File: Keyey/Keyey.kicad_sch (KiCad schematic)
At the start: 0 parts

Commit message: 22 July update
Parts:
- added A1: RaspberryPi_Pico_W, Module:RaspberryPi_Pico_W_SMD, symbol MCU_Module:RaspberryPi_Pico_W_Extensive
- added D1: Blue, LED_SMD:LED_0805_2012Metric_Pad1.15x1.40mm_HandSolder, symbol Device:LED
- added D10, D11, D12, D13, D14, D15, D16, D17, D18, D19, D2, D20, D21, D22, D23, D24, D25, D26, D27, D28, D29, D3, D30, D31, D32, D33, D34, D35, D36, D37, D38, D39, D40, D41, D42, D43, D44, D45, D46, D47, D48, D49, D50, D51, D52, D53, D54, D55, D56, D57, D58, D59, D6, D60, D61, D62, D63, D64, D65, D66, D67, D69, D70, D71, D74, D75, D76, D78, D79, D8, D80, D82, D83, D84, D85, D86, D87, D88, D89, D9, D90, D91, D92: 1N4148W, Diode_SMD:D_SOD-123, symbol Diode:1N4148W
- added D4: Red, LED_SMD:LED_0805_2012Metric_Pad1.15x1.40mm_HandSolder, symbol Device:LED
- added J1: USB_C_Receptacle_USB2.0_16P, Connector_USB:USB_C_Receptacle_Amphenol_12401948E412A, symbol Connector:USB_C_Receptacle_USB2.0_16P
- added J2: Conn_01x02_Pin, Connector_JST:JST_EH_S2B-EH_1x02_P2.50mm_Horizontal, symbol Connector:Conn_01x02_Pin
- added R1: 5.1K, Resistor_SMD:R_01005_0402Metric_Pad0.57x0.30mm_HandSolder, symbol Device:R
- added R2: 5.1k, Resistor_SMD:R_01005_0402Metric_Pad0.57x0.30mm_HandSolder, symbol Device:R
- added R3, R4: 27, Resistor_SMD:R_01005_0402Metric_Pad0.57x0.30mm_HandSolder, symbol Device:R
- added R5: 1.2K, Resistor_SMD:R_01005_0402Metric_Pad0.57x0.30mm_HandSolder, symbol Device:R
- added R6: 1+, Resistor_SMD:R_01005_0402Metric_Pad0.57x0.30mm_HandSolder, symbol Device:R
- added R7: 1-, Resistor_SMD:R_01005_0402Metric_Pad0.57x0.30mm_HandSolder, symbol Device:R
- added R8: 2+, Resistor_SMD:R_01005_0402Metric_Pad0.57x0.30mm_HandSolder, symbol Device:R
- added R9: 2-, Resistor_SMD:R_01005_0402Metric_Pad0.57x0.30mm_HandSolder, symbol Device:R
- added S1, S3, S4: Stab 2u, PCM_Mounting_Keyboard_Stabilizer:Stabilizer_Cherry_MX_2.00u, symbol PCM_marbastlib-mx:MX_stab
- added S2: Stab 6.25u, PCM_marbastlib-mx:STAB_MX_P_6.25u, symbol PCM_marbastlib-mx:MX_stab
- added SW1: EC11E15244G1, 2026-07-22_12-53-14:EC11E15244G1_AAL, symbol 2026-07-22_12-53-14:EC11E15244G1
- added SW10, SW89: Control, PCM_marbastlib-mx:SW_MX_1u, symbol Switch:SW_Push
- added SW11: F1, PCM_marbastlib-mx:SW_MX_1u, symbol Switch:SW_Push
- added SW12: 1, PCM_marbastlib-mx:SW_MX_1u, symbol Switch:SW_Push
- added SW13: Q, PCM_marbastlib-mx:SW_MX_1u, symbol Switch:SW_Push
- added SW14: A, PCM_marbastlib-mx:SW_MX_1u, symbol Switch:SW_Push
- added SW15: Z, PCM_marbastlib-mx:SW_MX_1u, symbol Switch:SW_Push
- added SW16: Win, PCM_marbastlib-mx:SW_MX_1u, symbol Switch:SW_Push
- added SW17: F2, PCM_marbastlib-mx:SW_MX_1u, symbol Switch:SW_Push
- added SW18: 2, PCM_marbastlib-mx:SW_MX_1u, symbol Switch:SW_Push
- added SW19: W, PCM_marbastlib-mx:SW_MX_1u, symbol Switch:SW_Push
- added SW2: Caplocks, PCM_marbastlib-mx:SW_MX_1u, symbol Switch:SW_Push
- added SW20: S, PCM_marbastlib-mx:SW_MX_1u, symbol Switch:SW_Push
- added SW21: X, PCM_marbastlib-mx:SW_MX_1u, symbol Switch:SW_Push
- added SW22: F3, PCM_marbastlib-mx:SW_MX_1u, symbol Switch:SW_Push
- added SW23: 3, PCM_marbastlib-mx:SW_MX_1u, symbol Switch:SW_Push
- added SW24: E, PCM_marbastlib-mx:SW_MX_1u, symbol Switch:SW_Push
- added SW25: D, PCM_marbastlib-mx:SW_MX_1u, symbol Switch:SW_Push
- added SW26: C, PCM_marbastlib-mx:SW_MX_1u, symbol Switch:SW_Push
- added SW27: F4, PCM_marbastlib-mx:SW_MX_1u, symbol Switch:SW_Push
- added SW28: 4, PCM_marbastlib-mx:SW_MX_1u, symbol Switch:SW_Push
- added SW29: R, PCM_marbastlib-mx:SW_MX_1u, symbol Switch:SW_Push
- added SW30: F, PCM_marbastlib-mx:SW_MX_1u, symbol Switch:SW_Push
- added SW31: V, PCM_marbastlib-mx:SW_MX_1u, symbol Switch:SW_Push
- added SW32, SW80: opt, PCM_marbastlib-mx:SW_MX_1u, symbol Switch:SW_Push
- added SW33: F5, PCM_marbastlib-mx:SW_MX_1u, symbol Switch:SW_Push
- added SW34: 5, PCM_marbastlib-mx:SW_MX_1u, symbol Switch:SW_Push
- added SW35: T, PCM_marbastlib-mx:SW_MX_1u, symbol Switch:SW_Push
- added SW36: G, PCM_marbastlib-mx:SW_MX_1u, symbol Switch:SW_Push
- added SW37: B, PCM_marbastlib-mx:SW_MX_1u, symbol Switch:SW_Push
- added SW38: F6, PCM_marbastlib-mx:SW_MX_1u, symbol Switch:SW_Push
- added SW39: 6, PCM_marbastlib-mx:SW_MX_1u, symbol Switch:SW_Push
- added SW4: Tab, PCM_marbastlib-mx:SW_MX_1u, symbol Switch:SW_Push
- added SW40: Y, PCM_marbastlib-mx:SW_MX_1u, symbol Switch:SW_Push
- added SW41: H, PCM_marbastlib-mx:SW_MX_1u, symbol Switch:SW_Push
- added SW42: N, PCM_marbastlib-mx:SW_MX_1u, symbol Switch:SW_Push
- added SW43: F7, PCM_marbastlib-mx:SW_MX_1u, symbol Switch:SW_Push
- added SW44: 7, PCM_marbastlib-mx:SW_MX_1u, symbol Switch:SW_Push
- added SW45: U, PCM_marbastlib-mx:SW_MX_1u, symbol Switch:SW_Push
- added SW46: J, PCM_marbastlib-mx:SW_MX_1u, symbol Switch:SW_Push
- added SW47: M, PCM_marbastlib-mx:SW_MX_1u, symbol Switch:SW_Push
- added SW48: Spacebar, PCM_marbastlib-mx:SW_MX_1u, symbol Switch:SW_Push
- added SW49: F8, PCM_marbastlib-mx:SW_MX_1u, symbol Switch:SW_Push
- added SW5: Left Shift, PCM_marbastlib-mx:SW_MX_1u, symbol Switch:SW_Push
- added SW50: 8, PCM_marbastlib-mx:SW_MX_1u, symbol Switch:SW_Push
- added SW51: I, PCM_marbastlib-mx:SW_MX_1u, symbol Switch:SW_Push
- added SW52: K, PCM_marbastlib-mx:SW_MX_1u, symbol Switch:SW_Push
- added SW53: ,, PCM_marbastlib-mx:SW_MX_1u, symbol Switch:SW_Push
- added SW54: F9, PCM_marbastlib-mx:SW_MX_1u, symbol Switch:SW_Push
- added SW55: 9, PCM_marbastlib-mx:SW_MX_1u, symbol Switch:SW_Push
- added SW56: O, PCM_marbastlib-mx:SW_MX_1u, symbol Switch:SW_Push
- added SW57: L, PCM_marbastlib-mx:SW_MX_1u, symbol Switch:SW_Push
- added SW58: ., PCM_marbastlib-mx:SW_MX_1u, symbol Switch:SW_Push
- added SW59: F10, PCM_marbastlib-mx:SW_MX_1u, symbol Switch:SW_Push
- added SW60: 0, PCM_marbastlib-mx:SW_MX_1u, symbol Switch:SW_Push
- added SW61: P, PCM_marbastlib-mx:SW_MX_1u, symbol Switch:SW_Push
- added SW62: ;, PCM_marbastlib-mx:SW_MX_1u, symbol Switch:SW_Push
- added SW63: /, PCM_marbastlib-mx:SW_MX_1u, symbol Switch:SW_Push
- added SW64: F11, PCM_marbastlib-mx:SW_MX_1u, symbol Switch:SW_Push
- added SW65: -, PCM_marbastlib-mx:SW_MX_1u, symbol Switch:SW_Push
- added SW66: [, PCM_marbastlib-mx:SW_MX_1u, symbol Switch:SW_Push
- added SW67: ', PCM_marbastlib-mx:SW_MX_1u, symbol Switch:SW_Push
- added SW69: F12, PCM_marbastlib-mx:SW_MX_1u, symbol Switch:SW_Push
- added SW70: =, PCM_marbastlib-mx:SW_MX_1u, symbol Switch:SW_Push
- added SW71: ], PCM_marbastlib-mx:SW_MX_1u, symbol Switch:SW_Push
- added SW74: prntsrc, PCM_marbastlib-mx:SW_MX_1u, symbol Switch:SW_Push
- added SW75: backspace, PCM_marbastlib-mx:SW_MX_1u, symbol Switch:SW_Push
- added SW76: \, PCM_marbastlib-mx:SW_MX_1u, symbol Switch:SW_Push
- added SW78: SHIFT, PCM_marbastlib-mx:SW_MX_1u, symbol Switch:SW_Push
- added SW79: del, PCM_marbastlib-mx:SW_MX_1u, symbol Switch:SW_Push
- added SW8: Esc, PCM_marbastlib-mx:SW_MX_1u, symbol Switch:SW_Push
- added SW82: ENTER, PCM_marbastlib-mx:SW_MX_1u, symbol Switch:SW_Push
- added SW83: up, PCM_marbastlib-mx:SW_MX_1u, symbol Switch:SW_Push
- added SW84: fn, PCM_marbastlib-mx:SW_MX_1u, symbol Switch:SW_Push
- added SW85: pgup, PCM_marbastlib-mx:SW_MX_1u, symbol Switch:SW_Push
- added SW86: pgdn, PCM_marbastlib-mx:SW_MX_1u, symbol Switch:SW_Push
- added SW87: home, PCM_marbastlib-mx:SW_MX_1u, symbol Switch:SW_Push
- added SW88: end, PCM_marbastlib-mx:SW_MX_1u, symbol Switch:SW_Push
- added SW9: ~, PCM_marbastlib-mx:SW_MX_1u, symbol Switch:SW_Push
- added SW90: left, PCM_marbastlib-mx:SW_MX_1u, symbol Switch:SW_Push
- added SW91: down, PCM_marbastlib-mx:SW_MX_1u, symbol Switch:SW_Push
- added SW92: right, PCM_marbastlib-mx:SW_MX_1u, symbol Switch:SW_Push
- added U1: TP4056, Package_SO:SOP-8-1EP_4.57x4.57mm_P1.27mm_EP4.57x4.45mm, symbol PCM_marbastlib-various:TP4056
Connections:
- new net: D91.2 (A), SW91.2
- new net: D24.2 (A), SW24.2
- new net: D29.2 (A), SW29.2
- new net: D46.2 (A), SW46.2
- new net: D89.2 (A), SW89.2
- new net: D83.2 (A), SW83.2
- new net: D90.2 (A), SW90.2
- new net: D65.2 (A), SW65.2
- new net: D70.2 (A), SW70.2
- new net: D15.2 (A), SW15.2
- new net: D82.2 (A), SW82.2
- new net: D14.2 (A), SW14.2
- new net: D76.2 (A), SW76.2
- new net: D10.2 (A), SW10.2
- new net: D26.2 (A), SW26.2
- new net: D42.2 (A), SW42.2
- new net: D37.2 (A), SW37.2
- new net: D39.2 (A), SW39.2
- new net: D6.2 (A), SW4.2
- new net: D13.2 (A), SW13.2
- new net: D87.2 (A), SW87.2
- new net: D51.2 (A), SW51.2
- new net: D12.2 (A), SW12.2
- new net: D20.2 (A), SW20.2
- new net: D11.2 (A), SW11.2
- new net: D22.2 (A), SW22.2
- new net: D57.2 (A), SW57.2
- new net: D48.2 (A), SW48.2
- new net: D80.2 (A), SW80.2
- new net: D85.2 (A), SW85.2
- new net: D21.2 (A), SW21.2
- new net: D67.2 (A), SW67.2
- new net: D36.2 (A), SW36.2
- new net: D50.2 (A), SW50.2
- new net: D9.2 (A), SW9.2
- new net: D55.2 (A), SW55.2
- new net: D64.2 (A), SW64.2
- new net: D2.2 (A), SW2.2
- new net: D17.2 (A), SW17.2
- new net: A1.40 (VBUS), J1.A4 (VBUS), J1.A9 (VBUS), J1.B4 (VBUS), J1.B9 (VBUS)
- new net: A1.TP2 (USB_DM), J1.A7 (D-), J1.B7 (D-), R3.2
- new net: A1.TP3 (USB_DP), J1.A6 (D+), J1.B6 (D+), R4.2
- new net: J1.B5 (CC2), R2.1
- new net: D66.2 (A), SW66.2
- new net: D79.2 (A), SW79.2
- new net: D75.2 (A), SW75.2
- new net: D23.2 (A), SW23.2
- new net: D88.2 (A), SW88.2
- new net: D61.2 (A), SW61.2
- new net: D71.2 (A), SW71.2
- new net: D31.2 (A), SW31.2
- new net: D25.2 (A), SW25.2
- new net: D30.2 (A), SW30.2
- new net: D18.2 (A), SW18.2
- new net: D8.2 (A), SW8.2
- new net: D33.2 (A), SW33.2
- new net: D54.2 (A), SW54.2
- new net: J2.1 (Pin_1), R6.1, R7.1
- new net: J2.2 (Pin_2), R8.2, R9.2
- new net: D62.2 (A), SW62.2
- new net: D86.2 (A), SW86.2
- new net: D19.2 (A), SW19.2
- new net: D32.2 (A), SW32.2
- new net: D43.2 (A), SW43.2
- new net: D40.2 (A), SW40.2
- new net: J1.A5 (CC1), R1.1
- new net: D53.2 (A), SW53.2
- new net: D35.2 (A), SW35.2
- new net: D34.2 (A), SW34.2
- new net: D3.2 (A), SW5.2
- new net: D58.2 (A), SW58.2
- new net: D60.2 (A), SW60.2
- new net: D52.2 (A), SW52.2
- new net: R6.2, R8.1, U1.5 (BAT)
- new net: D74.2 (A), SW74.2
- new net: R5.1, U1.2 (PROG)
- new net: D45.2 (A), SW45.2
- new net: D69.2 (A), SW69.2
- new net: D38.2 (A), SW38.2
- new net: D56.2 (A), SW56.2
- new net: D84.2 (A), SW84.2
- new net: R7.2, R9.1, U1.1 (TEMP)
- new net: D28.2 (A), SW28.2
- new net: D41.2 (A), SW41.2
- new net: D59.2 (A), SW59.2
- new net: D63.2 (A), SW63.2
- new net: D16.2 (A), SW16.2
- new net: D78.2 (A), SW78.2
- new net: D49.2 (A), SW49.2
- new net: D27.2 (A), SW27.2
- new net: D92.2 (A), SW92.2
- new net: D44.2 (A), SW44.2
- new net: D47.2 (A), SW47.2
- new net COL1: SW10.1, SW2.1, SW4.1, SW5.1, SW8.1, SW9.1
- new net COL10: SW54.1, SW55.1, SW56.1, SW57.1, SW58.1, SW80.1
- new net COL11: SW59.1, SW60.1, SW61.1, SW62.1, SW63.1, SW84.1
- new net COL12: SW64.1, SW65.1, SW66.1, SW67.1, SW78.1, SW90.1
- new net COL13: SW69.1, SW70.1, SW71.1, SW82.1, SW83.1, SW91.1
- new net COL14: SW74.1, SW75.1, SW76.1
- new net COL15: SW79.1, SW85.1, SW86.1, SW87.1, SW88.1, SW92.1
- new net COL2: SW11.1, SW12.1, SW13.1, SW14.1, SW15.1, SW16.1
- new net COL3: SW17.1, SW18.1, SW19.1, SW20.1, SW21.1, SW32.1
- new net COL4: SW22.1, SW23.1, SW24.1, SW25.1, SW26.1
- new net COL5: SW27.1, SW28.1, SW29.1, SW30.1, SW31.1
- new net COL6: SW33.1, SW34.1, SW35.1, SW36.1, SW37.1
- new net COL7: SW38.1, SW39.1, SW40.1, SW41.1, SW42.1
- new net COL8: SW43.1, SW44.1, SW45.1, SW46.1, SW47.1
- new net COL9: SW49.1, SW50.1, SW51.1, SW52.1, SW53.1
- new net GND: A1.13 (GND), A1.18 (GND), A1.23 (GND), A1.28 (GND), A1.3 (GND), A1.33 (AGND), A1.38 (GND), A1.8 (GND), A1.D2 (GND), A1.TP1 (USB_GND), J1.A1 (GND), J1.A12 (GND), J1.B1 (GND), J1.B12 (GND), J1.SH (SHIELD), R1.2, R2.2, R3.1, R4.1, R5.2
- new net ROW1: D11.1 (K), D17.1 (K), D22.1 (K), D27.1 (K), D33.1 (K), D38.1 (K), D43.1 (K), D49.1 (K), D54.1 (K), D59.1 (K), D64.1 (K), D69.1 (K), D74.1 (K), D79.1 (K), D8.1 (K)
- new net ROW2: D12.1 (K), D18.1 (K), D23.1 (K), D28.1 (K), D34.1 (K), D39.1 (K), D44.1 (K), D50.1 (K), D55.1 (K), D60.1 (K), D65.1 (K), D70.1 (K), D75.1 (K), D85.1 (K), D9.1 (K)
- new net ROW3: D13.1 (K), D19.1 (K), D24.1 (K), D29.1 (K), D35.1 (K), D40.1 (K), D45.1 (K), D51.1 (K), D56.1 (K), D6.1 (K), D61.1 (K), D66.1 (K), D71.1 (K), D76.1 (K), D86.1 (K)
- new net ROW4: D14.1 (K), D2.1 (K), D20.1 (K), D25.1 (K), D30.1 (K), D36.1 (K), D41.1 (K), D46.1 (K), D52.1 (K), D57.1 (K), D62.1 (K), D67.1 (K), D82.1 (K), D87.1 (K)
- new net ROW5: D15.1 (K), D21.1 (K), D26.1 (K), D3.1 (K), D31.1 (K), D37.1 (K), D42.1 (K), D47.1 (K), D53.1 (K), D58.1 (K), D63.1 (K), D83.1 (K), D88.1 (K)
- new net ROW6: D10.1 (K), D16.1 (K), D32.1 (K), D48.1 (K), D80.1 (K), D84.1 (K), D89.1 (K), D90.1 (K), D91.1 (K), D92.1 (K)

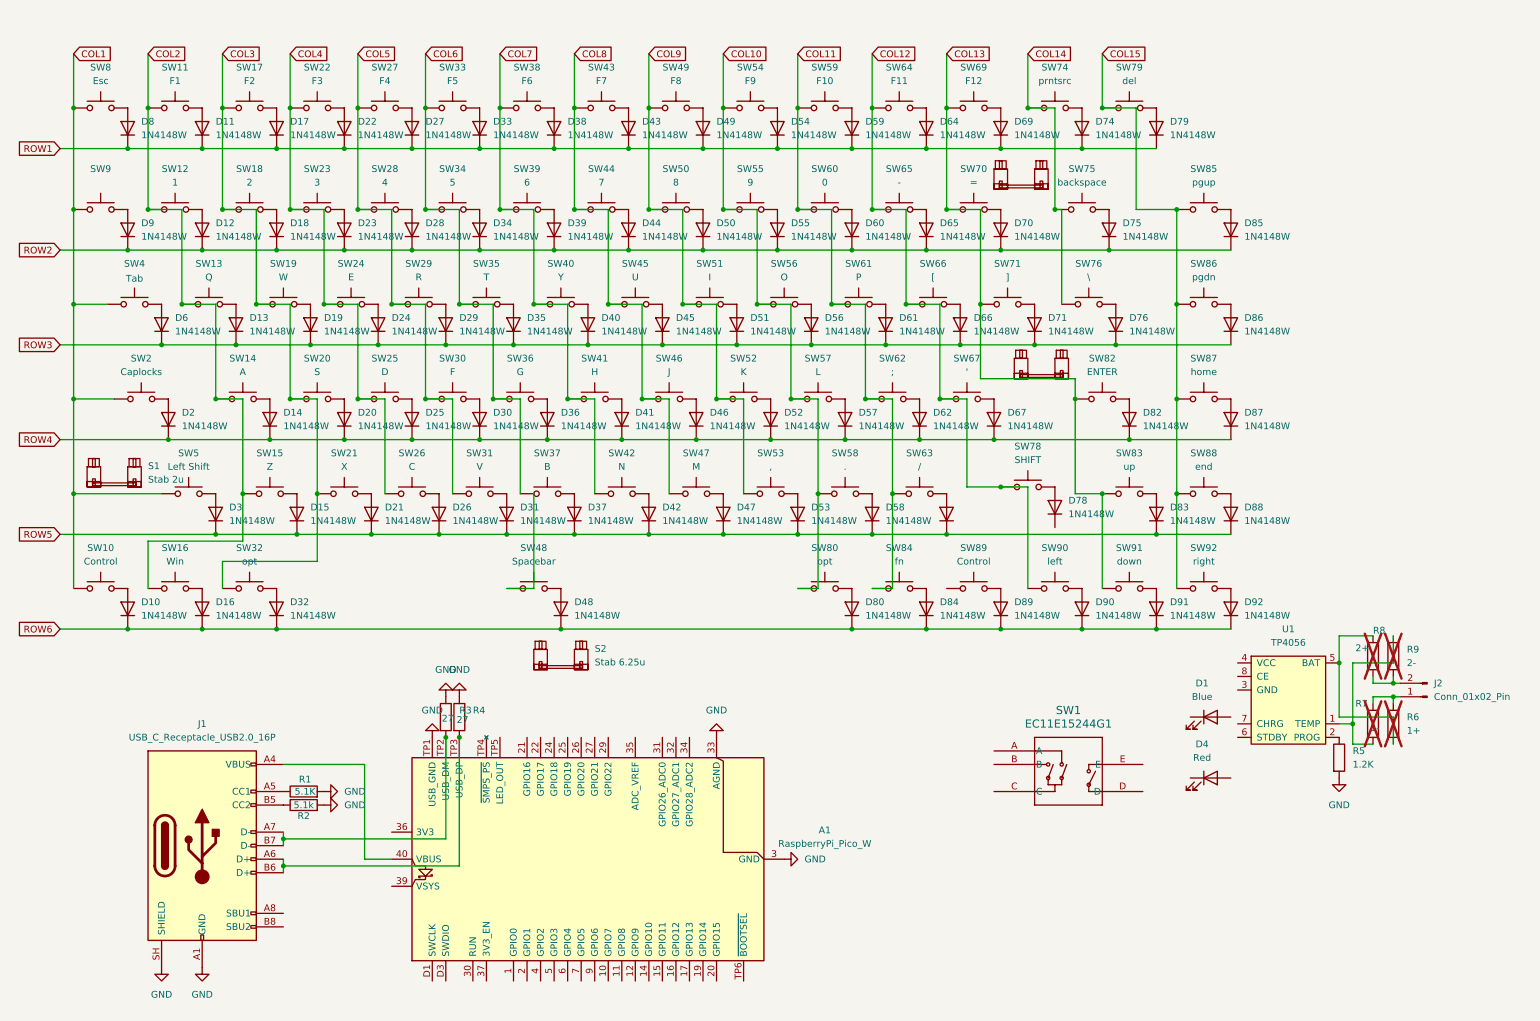
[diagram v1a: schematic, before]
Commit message: July 23-25 update
More info check: https://stardance.hackclub.com/projects/10369
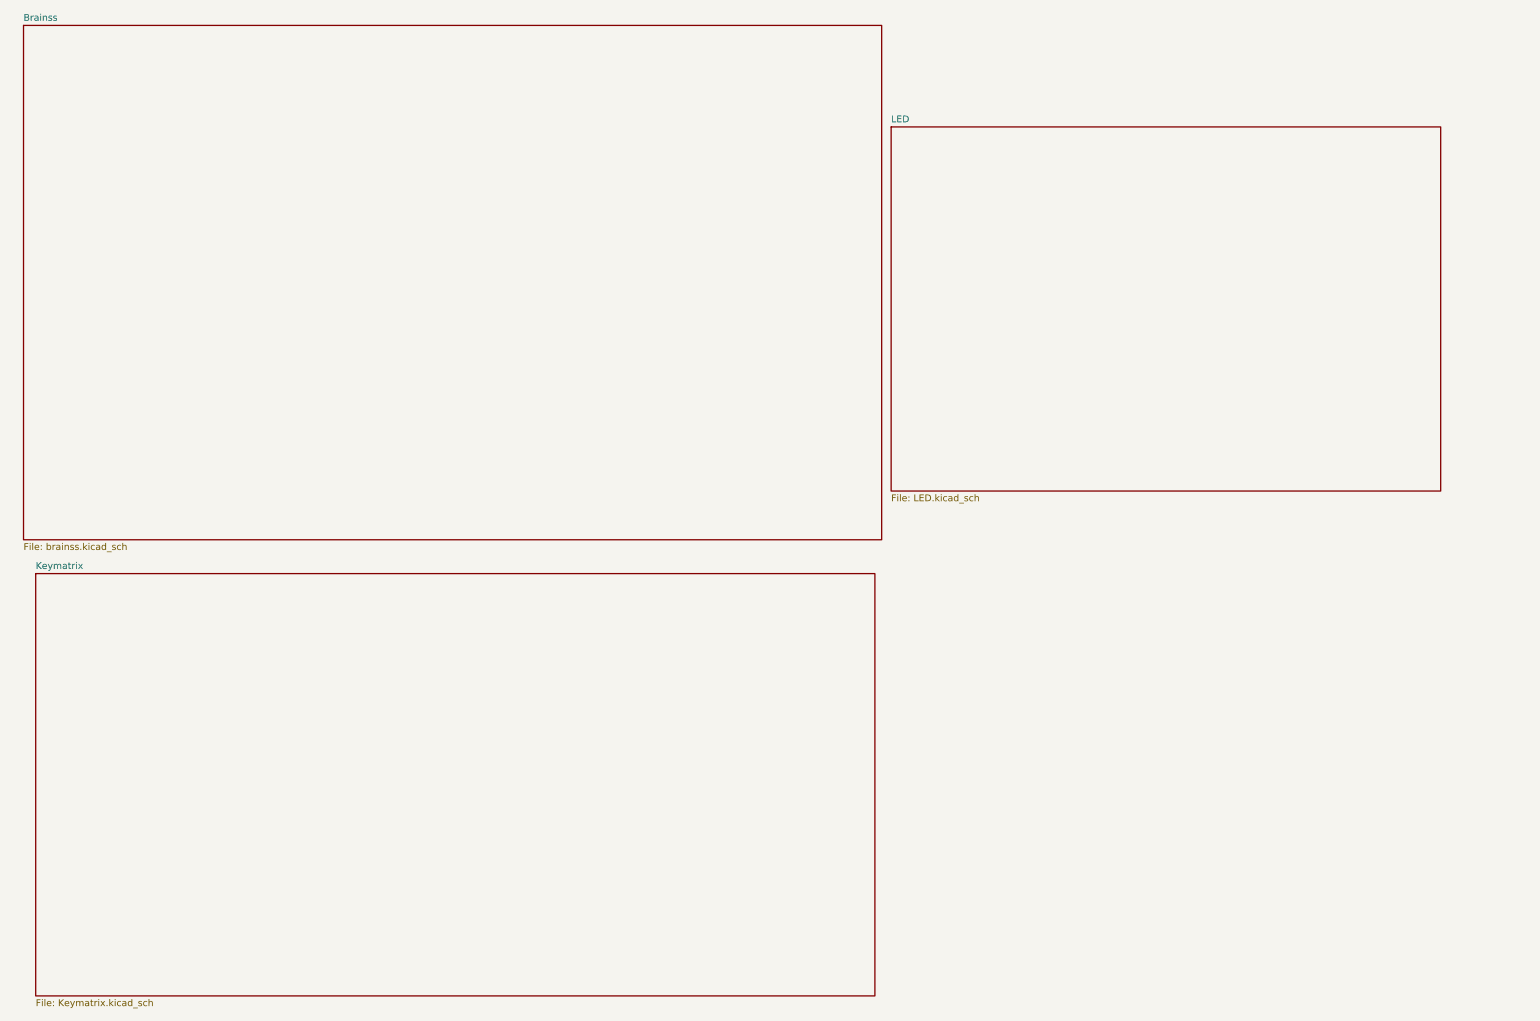
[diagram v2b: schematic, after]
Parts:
- removed A1: RaspberryPi_Pico_W, Module:RaspberryPi_Pico_W_SMD, symbol MCU_Module:RaspberryPi_Pico_W_Extensive
- removed D1: Blue, LED_SMD:LED_0805_2012Metric_Pad1.15x1.40mm_HandSolder, symbol Device:LED
- removed D10, D11, D12, D13, D14, D15, D16, D17, D18, D19, D2, D20, D21, D22, D23, D24, D25, D26, D27, D28, D29, D3, D30, D31, D32, D33, D34, D35, D36, D37, D38, D39, D40, D41, D42, D43, D44, D45, D46, D47, D48, D49, D50, D51, D52, D53, D54, D55, D56, D57, D58, D59, D6, D60, D61, D62, D63, D64, D65, D66, D67, D69, D70, D71, D74, D75, D76, D78, D79, D8, D80, D82, D83, D84, D85, D86, D87, D88, D89, D9, D90, D91, D92: 1N4148W, Diode_SMD:D_SOD-123, symbol Diode:1N4148W
- removed D4: Red, LED_SMD:LED_0805_2012Metric_Pad1.15x1.40mm_HandSolder, symbol Device:LED
- removed J1: USB_C_Receptacle_USB2.0_16P, Connector_USB:USB_C_Receptacle_Amphenol_12401948E412A, symbol Connector:USB_C_Receptacle_USB2.0_16P
- removed J2: Conn_01x02_Pin, Connector_JST:JST_EH_S2B-EH_1x02_P2.50mm_Horizontal, symbol Connector:Conn_01x02_Pin
- removed R1: 5.1K, Resistor_SMD:R_01005_0402Metric_Pad0.57x0.30mm_HandSolder, symbol Device:R
- removed R2: 5.1k, Resistor_SMD:R_01005_0402Metric_Pad0.57x0.30mm_HandSolder, symbol Device:R
- removed R3, R4: 27, Resistor_SMD:R_01005_0402Metric_Pad0.57x0.30mm_HandSolder, symbol Device:R
- removed R5: 1.2K, Resistor_SMD:R_01005_0402Metric_Pad0.57x0.30mm_HandSolder, symbol Device:R
- removed R6: 1+, Resistor_SMD:R_01005_0402Metric_Pad0.57x0.30mm_HandSolder, symbol Device:R
- removed R7: 1-, Resistor_SMD:R_01005_0402Metric_Pad0.57x0.30mm_HandSolder, symbol Device:R
- removed R8: 2+, Resistor_SMD:R_01005_0402Metric_Pad0.57x0.30mm_HandSolder, symbol Device:R
- removed R9: 2-, Resistor_SMD:R_01005_0402Metric_Pad0.57x0.30mm_HandSolder, symbol Device:R
- removed S1, S3, S4: Stab 2u, PCM_Mounting_Keyboard_Stabilizer:Stabilizer_Cherry_MX_2.00u, symbol PCM_marbastlib-mx:MX_stab
- removed S2: Stab 6.25u, PCM_marbastlib-mx:STAB_MX_P_6.25u, symbol PCM_marbastlib-mx:MX_stab
- removed SW1: EC11E15244G1, 2026-07-22_12-53-14:EC11E15244G1_AAL, symbol 2026-07-22_12-53-14:EC11E15244G1
- removed SW10, SW89: Control, PCM_marbastlib-mx:SW_MX_1u, symbol Switch:SW_Push
- removed SW11: F1, PCM_marbastlib-mx:SW_MX_1u, symbol Switch:SW_Push
- removed SW12: 1, PCM_marbastlib-mx:SW_MX_1u, symbol Switch:SW_Push
- removed SW13: Q, PCM_marbastlib-mx:SW_MX_1u, symbol Switch:SW_Push
- removed SW14: A, PCM_marbastlib-mx:SW_MX_1u, symbol Switch:SW_Push
- removed SW15: Z, PCM_marbastlib-mx:SW_MX_1u, symbol Switch:SW_Push
- removed SW16: Win, PCM_marbastlib-mx:SW_MX_1u, symbol Switch:SW_Push
- removed SW17: F2, PCM_marbastlib-mx:SW_MX_1u, symbol Switch:SW_Push
- removed SW18: 2, PCM_marbastlib-mx:SW_MX_1u, symbol Switch:SW_Push
- removed SW19: W, PCM_marbastlib-mx:SW_MX_1u, symbol Switch:SW_Push
- removed SW2: Caplocks, PCM_marbastlib-mx:SW_MX_1u, symbol Switch:SW_Push
- removed SW20: S, PCM_marbastlib-mx:SW_MX_1u, symbol Switch:SW_Push
- removed SW21: X, PCM_marbastlib-mx:SW_MX_1u, symbol Switch:SW_Push
- removed SW22: F3, PCM_marbastlib-mx:SW_MX_1u, symbol Switch:SW_Push
- removed SW23: 3, PCM_marbastlib-mx:SW_MX_1u, symbol Switch:SW_Push
- removed SW24: E, PCM_marbastlib-mx:SW_MX_1u, symbol Switch:SW_Push
- removed SW25: D, PCM_marbastlib-mx:SW_MX_1u, symbol Switch:SW_Push
- removed SW26: C, PCM_marbastlib-mx:SW_MX_1u, symbol Switch:SW_Push
- removed SW27: F4, PCM_marbastlib-mx:SW_MX_1u, symbol Switch:SW_Push
- removed SW28: 4, PCM_marbastlib-mx:SW_MX_1u, symbol Switch:SW_Push
- removed SW29: R, PCM_marbastlib-mx:SW_MX_1u, symbol Switch:SW_Push
- removed SW30: F, PCM_marbastlib-mx:SW_MX_1u, symbol Switch:SW_Push
- removed SW31: V, PCM_marbastlib-mx:SW_MX_1u, symbol Switch:SW_Push
- removed SW32, SW80: opt, PCM_marbastlib-mx:SW_MX_1u, symbol Switch:SW_Push
- removed SW33: F5, PCM_marbastlib-mx:SW_MX_1u, symbol Switch:SW_Push
- removed SW34: 5, PCM_marbastlib-mx:SW_MX_1u, symbol Switch:SW_Push
- removed SW35: T, PCM_marbastlib-mx:SW_MX_1u, symbol Switch:SW_Push
- removed SW36: G, PCM_marbastlib-mx:SW_MX_1u, symbol Switch:SW_Push
- removed SW37: B, PCM_marbastlib-mx:SW_MX_1u, symbol Switch:SW_Push
- removed SW38: F6, PCM_marbastlib-mx:SW_MX_1u, symbol Switch:SW_Push
- removed SW39: 6, PCM_marbastlib-mx:SW_MX_1u, symbol Switch:SW_Push
- removed SW4: Tab, PCM_marbastlib-mx:SW_MX_1u, symbol Switch:SW_Push
- removed SW40: Y, PCM_marbastlib-mx:SW_MX_1u, symbol Switch:SW_Push
- removed SW41: H, PCM_marbastlib-mx:SW_MX_1u, symbol Switch:SW_Push
- removed SW42: N, PCM_marbastlib-mx:SW_MX_1u, symbol Switch:SW_Push
- removed SW43: F7, PCM_marbastlib-mx:SW_MX_1u, symbol Switch:SW_Push
- removed SW44: 7, PCM_marbastlib-mx:SW_MX_1u, symbol Switch:SW_Push
- removed SW45: U, PCM_marbastlib-mx:SW_MX_1u, symbol Switch:SW_Push
- removed SW46: J, PCM_marbastlib-mx:SW_MX_1u, symbol Switch:SW_Push
- removed SW47: M, PCM_marbastlib-mx:SW_MX_1u, symbol Switch:SW_Push
- removed SW48: Spacebar, PCM_marbastlib-mx:SW_MX_1u, symbol Switch:SW_Push
- removed SW49: F8, PCM_marbastlib-mx:SW_MX_1u, symbol Switch:SW_Push
- removed SW5: Left Shift, PCM_marbastlib-mx:SW_MX_1u, symbol Switch:SW_Push
- removed SW50: 8, PCM_marbastlib-mx:SW_MX_1u, symbol Switch:SW_Push
- removed SW51: I, PCM_marbastlib-mx:SW_MX_1u, symbol Switch:SW_Push
- removed SW52: K, PCM_marbastlib-mx:SW_MX_1u, symbol Switch:SW_Push
- removed SW53: ,, PCM_marbastlib-mx:SW_MX_1u, symbol Switch:SW_Push
- removed SW54: F9, PCM_marbastlib-mx:SW_MX_1u, symbol Switch:SW_Push
- removed SW55: 9, PCM_marbastlib-mx:SW_MX_1u, symbol Switch:SW_Push
- removed SW56: O, PCM_marbastlib-mx:SW_MX_1u, symbol Switch:SW_Push
- removed SW57: L, PCM_marbastlib-mx:SW_MX_1u, symbol Switch:SW_Push
- removed SW58: ., PCM_marbastlib-mx:SW_MX_1u, symbol Switch:SW_Push
- removed SW59: F10, PCM_marbastlib-mx:SW_MX_1u, symbol Switch:SW_Push
- removed SW60: 0, PCM_marbastlib-mx:SW_MX_1u, symbol Switch:SW_Push
- removed SW61: P, PCM_marbastlib-mx:SW_MX_1u, symbol Switch:SW_Push
- removed SW62: ;, PCM_marbastlib-mx:SW_MX_1u, symbol Switch:SW_Push
- removed SW63: /, PCM_marbastlib-mx:SW_MX_1u, symbol Switch:SW_Push
- removed SW64: F11, PCM_marbastlib-mx:SW_MX_1u, symbol Switch:SW_Push
- removed SW65: -, PCM_marbastlib-mx:SW_MX_1u, symbol Switch:SW_Push
- removed SW66: [, PCM_marbastlib-mx:SW_MX_1u, symbol Switch:SW_Push
- removed SW67: ', PCM_marbastlib-mx:SW_MX_1u, symbol Switch:SW_Push
- removed SW69: F12, PCM_marbastlib-mx:SW_MX_1u, symbol Switch:SW_Push
- removed SW70: =, PCM_marbastlib-mx:SW_MX_1u, symbol Switch:SW_Push
- removed SW71: ], PCM_marbastlib-mx:SW_MX_1u, symbol Switch:SW_Push
- removed SW74: prntsrc, PCM_marbastlib-mx:SW_MX_1u, symbol Switch:SW_Push
- removed SW75: backspace, PCM_marbastlib-mx:SW_MX_1u, symbol Switch:SW_Push
- removed SW76: \, PCM_marbastlib-mx:SW_MX_1u, symbol Switch:SW_Push
- removed SW78: SHIFT, PCM_marbastlib-mx:SW_MX_1u, symbol Switch:SW_Push
- removed SW79: del, PCM_marbastlib-mx:SW_MX_1u, symbol Switch:SW_Push
- removed SW8: Esc, PCM_marbastlib-mx:SW_MX_1u, symbol Switch:SW_Push
- removed SW82: ENTER, PCM_marbastlib-mx:SW_MX_1u, symbol Switch:SW_Push
- removed SW83: up, PCM_marbastlib-mx:SW_MX_1u, symbol Switch:SW_Push
- removed SW84: fn, PCM_marbastlib-mx:SW_MX_1u, symbol Switch:SW_Push
- removed SW85: pgup, PCM_marbastlib-mx:SW_MX_1u, symbol Switch:SW_Push
- removed SW86: pgdn, PCM_marbastlib-mx:SW_MX_1u, symbol Switch:SW_Push
- removed SW87: home, PCM_marbastlib-mx:SW_MX_1u, symbol Switch:SW_Push
- removed SW88: end, PCM_marbastlib-mx:SW_MX_1u, symbol Switch:SW_Push
- removed SW9: ~, PCM_marbastlib-mx:SW_MX_1u, symbol Switch:SW_Push
- removed SW90: left, PCM_marbastlib-mx:SW_MX_1u, symbol Switch:SW_Push
- removed SW91: down, PCM_marbastlib-mx:SW_MX_1u, symbol Switch:SW_Push
- removed SW92: right, PCM_marbastlib-mx:SW_MX_1u, symbol Switch:SW_Push
- removed U1: TP4056, Package_SO:SOP-8-1EP_4.57x4.57mm_P1.27mm_EP4.57x4.45mm, symbol PCM_marbastlib-various:TP4056
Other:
- added sheet Brainss (brainss.kicad_sch)
- added sheet Keymatrix (Keymatrix.kicad_sch)
- added sheet LED (LED.kicad_sch)
